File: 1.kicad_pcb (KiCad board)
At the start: 2 copper layers, 85.1 x 45.7 mm, 52 parts, among them J1 USB_B_Micro, J10 SPI2, J11 Micro_SD_Card, J12 Conn_01x04, J2 Power, J3 SWD, J4 Conn_01x02, J5 ADC, J6 SPI1, J7 UART1, J8 BxI2C1, J9 Conn_01x04, K1 NRST, K2 WKUP, K3 KPA0, U1 STM32F103C8Tx, U2 AMS1117-3.3, Y1 8MHz, Y2 32.768k

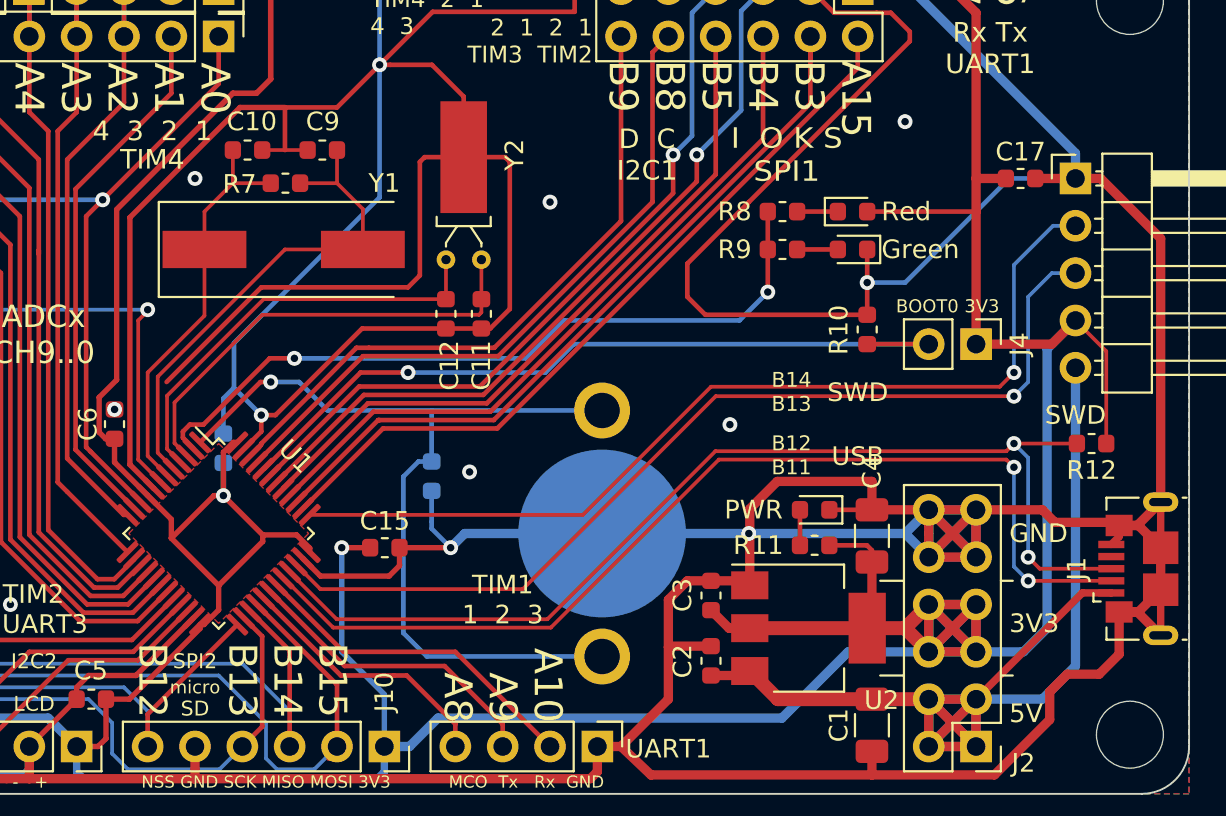
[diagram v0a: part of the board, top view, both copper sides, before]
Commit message: 视频中修改
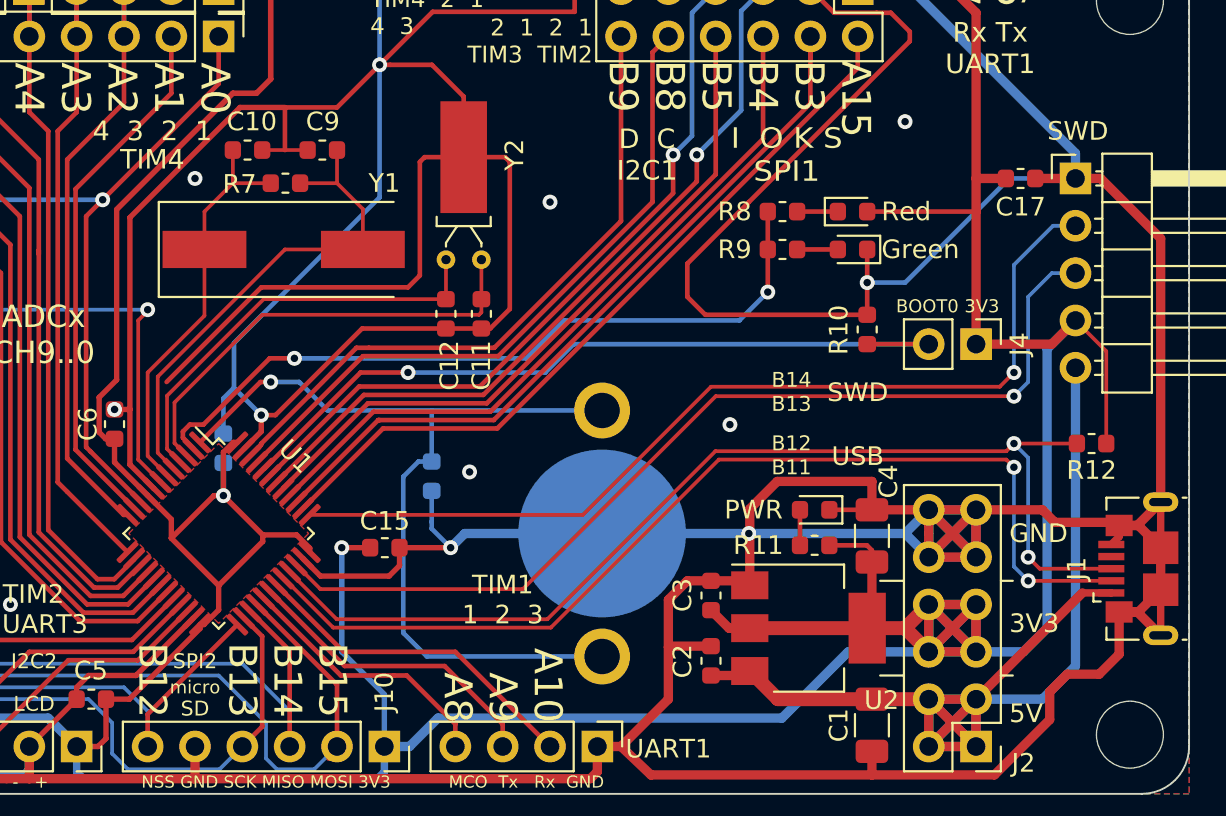
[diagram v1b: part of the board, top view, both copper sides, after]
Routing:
- net GND: track 702.8 -> 703.6 mm
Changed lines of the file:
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@@
     (thickness 1.6)
     (drawings 83)
-    (tracks 772)
+    (tracks 775)
     (zones 0)
     (modules 52)
@@
   )
   (setup
-    (last_trace_width 0.25)
+    (last_trace_width 0.29)
     (user_trace_width 0.2)
     (user_trace_width 0.29)
@@
     (tags capacitor)
     (attr smd)
-    (fp_text reference C17 (at 0 -1.43) (layer F.SilkS)
+    (fp_text reference C17 (at 0 1.524) (layer F.SilkS)
       (effects (font (size 1 1) (thickness 0.15)))
     )
@@
     (tags capacitor)
     (attr smd)
-    (fp_text reference C4 (at 3.432 0 90) (layer F.SilkS)
+    (fp_text reference C4 (at 2.924 0.889 90) (layer F.SilkS)
       (effects (font (size 1 1) (thickness 0.15)))
     )
@@
     (effects (font (size 1 1) (thickness 0.15)) (justify left))
   )
-  (gr_text SWD (at 175.514 111.76) (layer F.SilkS)
+  (gr_text SWD (at 175.641 96.52) (layer F.SilkS)
     (effects (font (size 1 1) (thickness 0.2)))
   )
@@
   (segment (start 140.335 98.171) (end 140.335 104.267) (width 0.25) (layer F.Cu) (net 2))
   (segment (start 133.096 95.25) (end 133.096 97.536) (width 0.25) (layer F.Cu) (net 2))
-  (segment (start 131.826 112.64202) (end 130.892342 113.575678) (width 0.25) (layer F.Cu) (net 2))
+  (segment (start 131.826 112.64202) (end 130.892342 113.575678) (width 0.29) (layer F.Cu) (net 2))
   (segment (start 132.588 111.76) (end 131.826 111.76) (width 0.25) (layer F.Cu) (net 2))
   (segment (start 137.236 107.112) (end 132.588 111.76) (width 0.25) (layer F.Cu) (net 2))
   (segment (start 131.826 111.76) (end 131.826 111.76) (width 0.25) (layer F.Cu) (net 2))
   (segment (start 141.732 107.112) (end 137.236 107.112) (width 0.25) (layer F.Cu) (net 2))
-  (segment (start 131.826 111.76) (end 131.826 112.64202) (width 0.25) (layer F.Cu) (net 2))
+  (segment (start 131.826 111.76) (end 131.826 112.64202) (width 0.29) (layer F.Cu) (net 2))
   (via (at 131.826 111.76) (size 0.8) (drill 0.4) (layers F.Cu B.Cu) (net 2))
   (segment (start 130.359685 110.293685) (end 131.826 111.76) (width 0.25) (layer B.Cu) (net 2))
@@
   (segment (start 130.683 95.25) (end 133.096 95.25) (width 0.29) (layer F.Cu) (net 2))
   (segment (start 124.77699 101.15601) (end 130.683 95.25) (width 0.29) (layer F.Cu) (net 2))
-  (segment (start 124.77699 114.414704) (end 124.77699 101.15601) (width 0.29) (layer F.Cu) (net 2))
   (segment (start 126.059284 115.696998) (end 124.77699 114.414704) (width 0.29) (layer F.Cu) (net 2))
   (segment (start 126.066338 115.696998) (end 126.059284 115.696998) (width 0.29) (layer F.Cu) (net 2))
@@
   (segment (start 142.687 94.667) (end 140.984 92.964) (width 0.25) (layer F.Cu) (net 2))
   (segment (start 142.687 97.917) (end 142.687 94.667) (width 0.25) (layer F.Cu) (net 2))
+  (segment (start 124.765 111.455) (end 123.952 111.455) (width 0.29) (layer F.Cu) (net 2))
+  (segment (start 124.77699 111.44301) (end 124.765 111.455) (width 0.29) (layer F.Cu) (net 2))
+  (segment (start 124.77699 114.414704) (end 124.77699 111.44301) (width 0.29) (layer F.Cu) (net 2))
+  (segment (start 124.77699 111.44301) (end 124.77699 101.15601) (width 0.29) (layer F.Cu) (net 2))
   (segment (start 170.18 100.838) (end 170.18 107.95) (width 0.5) (layer F.Cu) (net 3))
   (segment (start 125.712785 116.060785) (end 125.712785 116.050551) (width 0.25) (layer F.Cu) (net 3))
@@
   (segment (start 177.433 121.297) (end 177.436 121.3) (width 0.4) (layer F.Cu) (net 4))
   (segment (start 175.883 121.297) (end 177.433 121.297) (width 0.4) (layer F.Cu) (net 4))
-  (segment (start 170.18 127) (end 175.883 121.297) (width 0.4) (layer F.Cu) (net 4))
+  (segment (start 170.18 127) (end 175.883 121.297) (width 0.5) (layer F.Cu) (net 4))
   (segment (start 159.548 127) (end 158.038 125.49) (width 0.75) (layer F.Cu) (net 4))
   (segment (start 164.592 127) (end 159.548 127) (width 0.75) (layer F.Cu) (net 4))

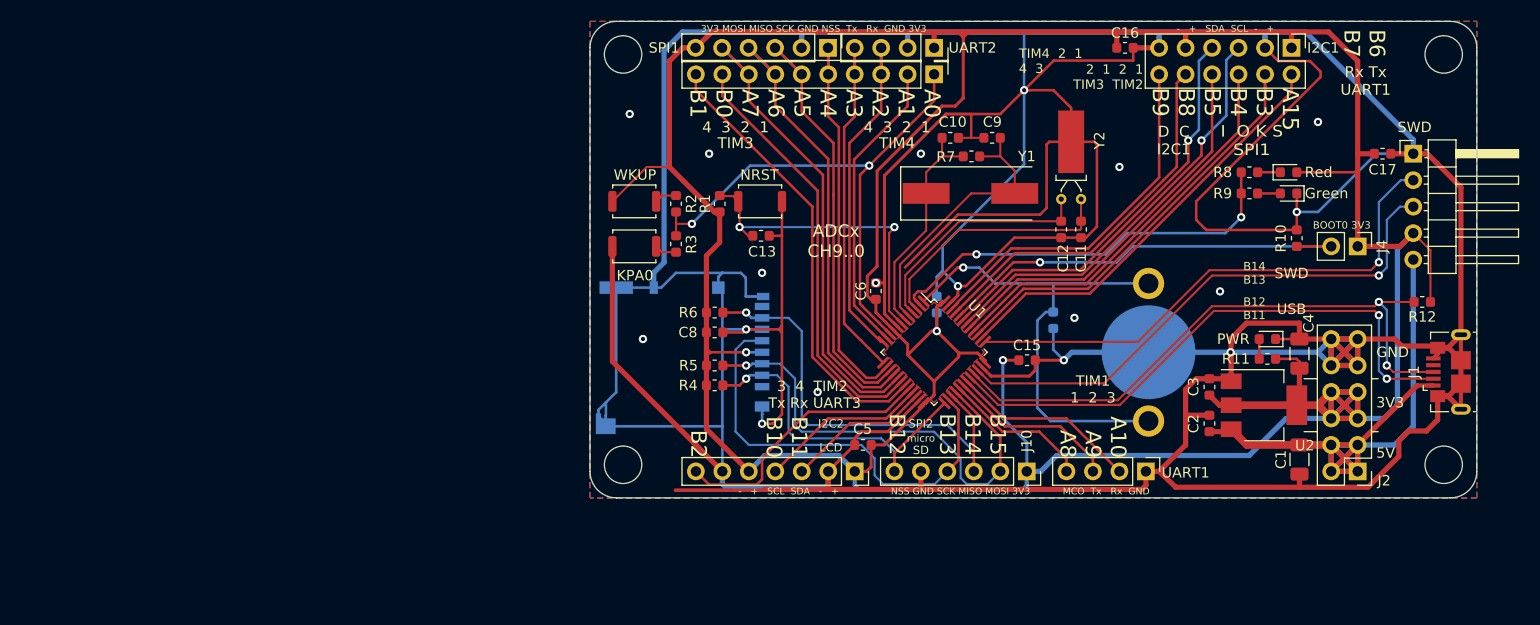
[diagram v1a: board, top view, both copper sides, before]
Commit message: tran 90deg
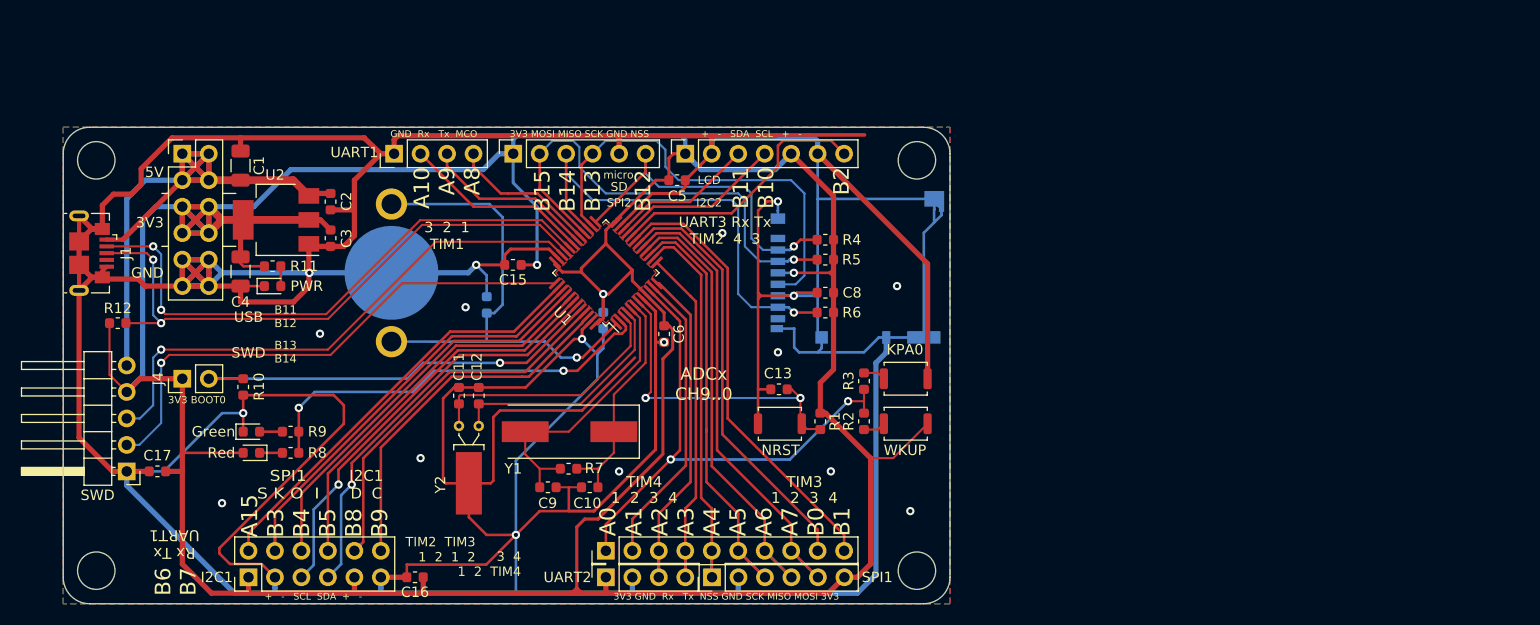
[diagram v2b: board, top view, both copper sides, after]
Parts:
- moved J1 130.7 mm to (48.7, 108.6), turned to 270 degrees
- moved J3 127.2 mm to (52.1, 129.5), turned to 180 degrees
- moved R12 125.2 mm to (51.2, 115.3), turned to 0 degrees
- moved C17 121.4 mm to (55.0, 129.5), turned to 180 degrees
- moved J2 116.8 mm to (57.4, 99.1), turned to 0 degrees
- moved J4 113.5 mm to (57.4, 120.7), turned to 90 degrees
- moved J8 112.2 mm to (63.8, 139.7), turned to 90 degrees
- moved C1 105.4 mm to (63.0, 100.2), turned to 90 degrees
- moved D1 103.1 mm to (64.0, 127.8), turned to 180 degrees
- moved D2 102.1 mm to (64.0, 125.7), turned to 0 degrees
- moved R10 102.1 mm to (63.2, 121.4), turned to 270 degrees
- moved C4 101.9 mm to (63.0, 110.4), turned to 270 degrees
- moved U2 96.4 mm to (66.4, 105.4), turned to 180 degrees
- moved R11 95.9 mm to (66.1, 109.9), turned to 0 degrees
- moved R8 95.9 mm to (67.8, 127.8), turned to 0 degrees
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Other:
- outline, holes or cut-outs redrawn
- board text added: "+ - SCL SDA + -"
- board text added: "+ - SDA SCL + -"
- board text added: "1 2 3 4"
- board text added: "3 2 1 TIM1"
- board text added: "3 4 1 2 TIM4"
- board text added: "3V3 GND Rx Tx NSS GND SCK MISO MOSI 3V3"
- board text added: "3V3 MOSI MISO SCK GND NSS"
- board text added: "5V 3V3 GND"
- board text added: "B11 B12"
- board text added: "B13 B14"
- board text added: "GND Rx Tx MCO"
- board text added: "I2C1 D C"
- board text added: "SPI1 S K O I"
- board text added: "TIM2 TIM3 1 2 1 2"
- board text added: "UART3 Rx Tx TIM2 4 3"
- board text removed: "- + SCL SDA - +"
- board text removed: "- + SDA SCL - +"
- board text removed: "2 1 2 1 TIM3 TIM2"
- board text removed: "3 4 TIM2 Tx Rx UART3"
- board text removed: "3V3 MOSI MISO SCK GND NSS Tx Rx GND 3V3"
- board text removed: "4 3 2 1"
- board text removed: "B12 B11"
- board text removed: "B14 B13"
- board text removed: "BOOT0 3V3"
- board text removed: "D C I2C1"
- board text removed: "I O K S SPI1"
- board text removed: "MCO Tx Rx GND"
- board text removed: "NSS GND SCK MISO MOSI 3V3"
- board text removed: "TIM1 1 2 3"
- board text removed: "TIM4 2 1 4 3"

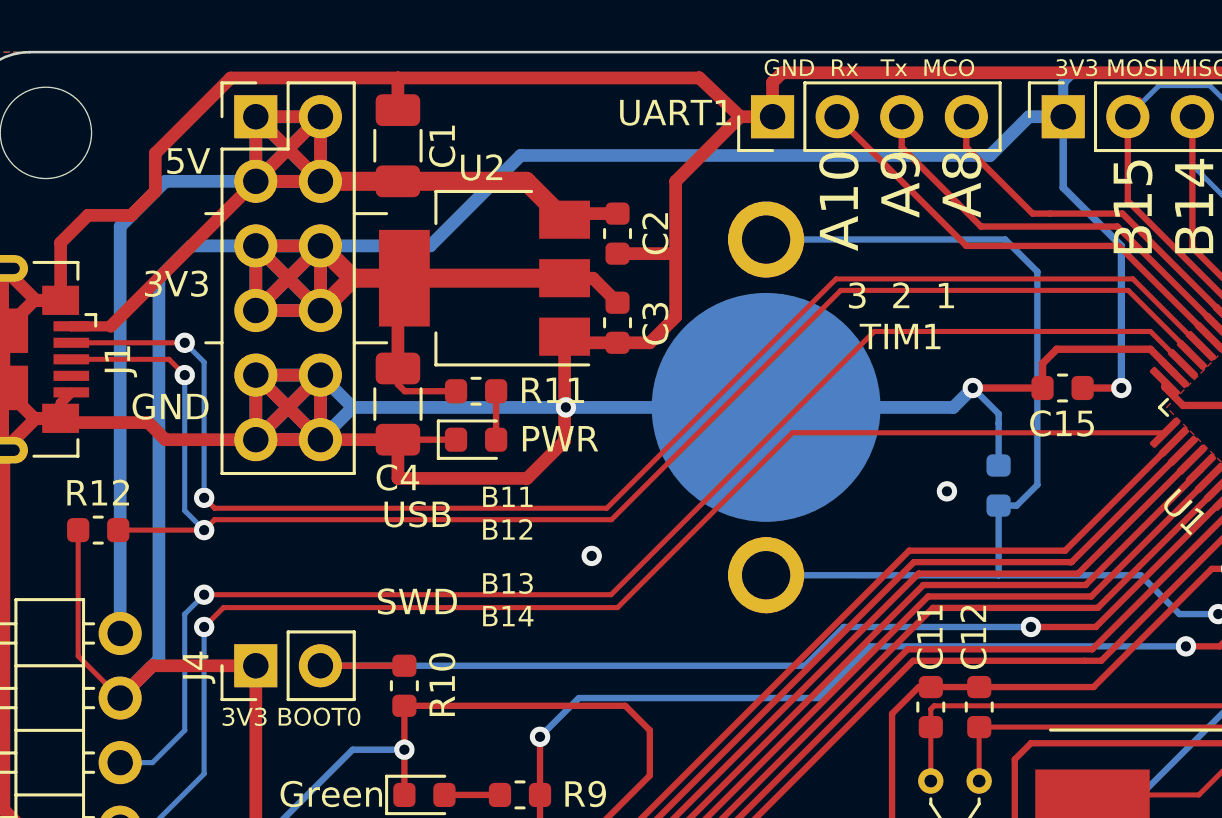
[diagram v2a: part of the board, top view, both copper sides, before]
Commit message: lines near power PinHeader
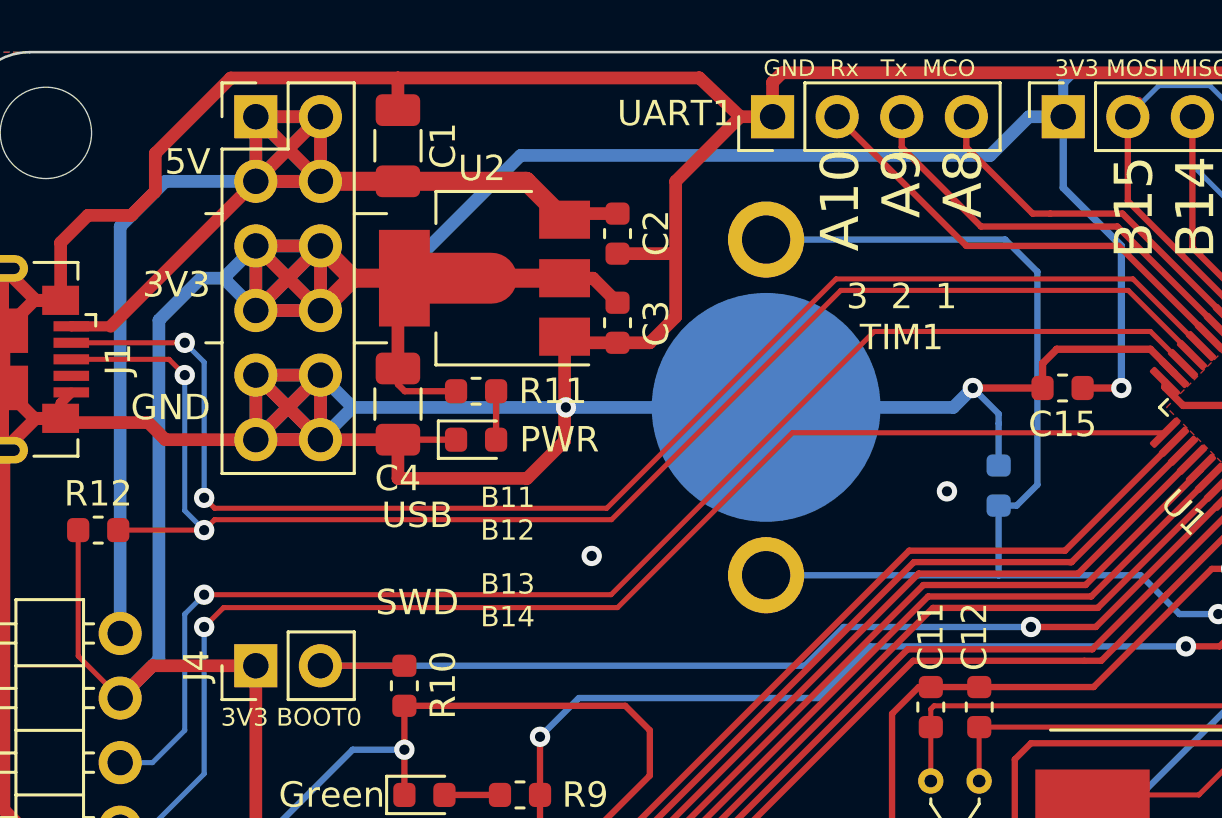
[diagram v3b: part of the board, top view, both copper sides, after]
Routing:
- net +3V3: track 397.3 -> 401.0 mm
